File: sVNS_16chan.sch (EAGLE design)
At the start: 56 parts, among them IC2 OPA990IDCKR, IC3 EFM8SB10F2G-A-QFN20, J1 M50-3631042, J2 M50-3631042, J3 M50-3631042, U1 NT3H2211W0FHKH, U2 LT8410EDC-1#TRMPBF, U3 MUX36S16IRSNR, U4 MUX36S16IRSNR

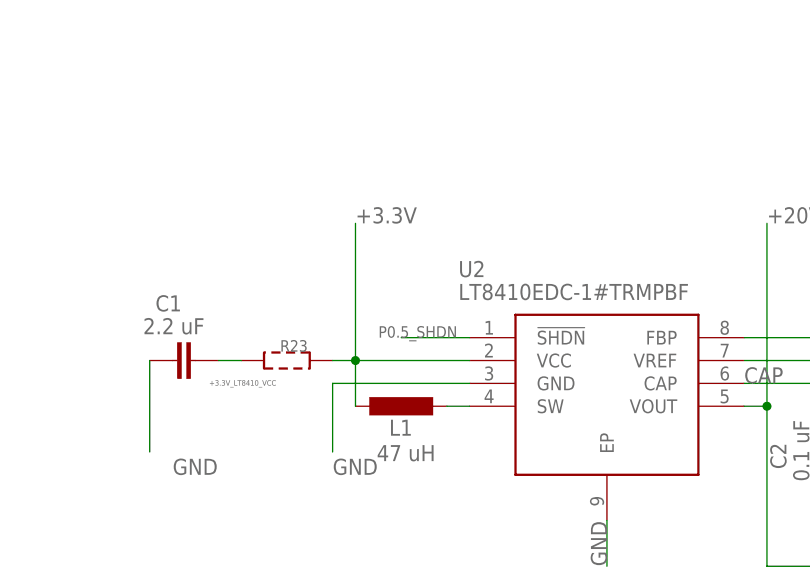
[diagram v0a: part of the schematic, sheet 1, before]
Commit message: Checkpoint 5. Closer to success?
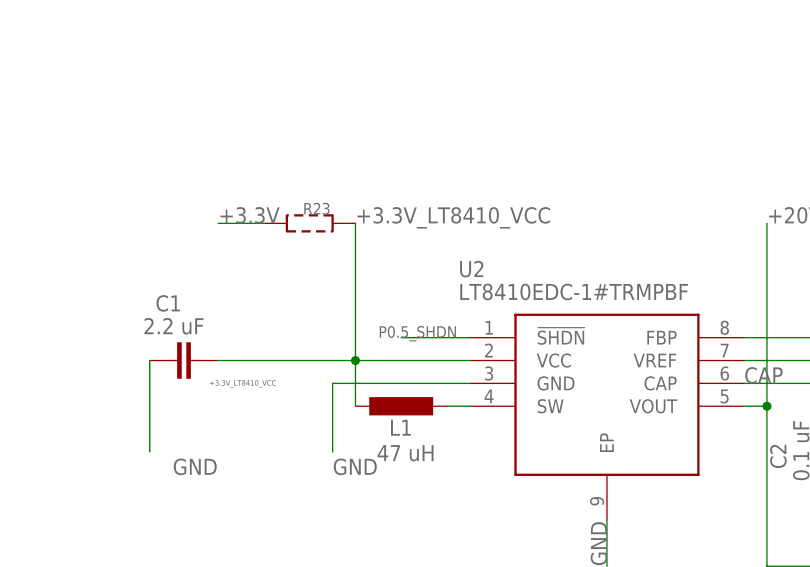
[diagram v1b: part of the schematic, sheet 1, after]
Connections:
- net +3.3V: now also R23.1; no longer L1.1, R23.2, U2.VCC
- net +3.3V_LT8410_VCC: now also L1.1, R23.2, U2.VCC; no longer R23.1
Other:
- moved on the sheet: R23
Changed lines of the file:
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@@
 <part name="R19" library="sVNS_16chan_lib" deviceset="SMD_PADS_0603" device="" package3d_urn="urn:adsk.eagle:package:23555/3"/>
 <part name="R20" library="sVNS_16chan_lib" deviceset="SMD_PADS_0603" device="" package3d_urn="urn:adsk.eagle:package:23555/3"/>
-<part name="R23" library="sVNS_16chan_lib" deviceset="SMD_PADS_0603" device="" package3d_urn="urn:adsk.eagle:package:23555/3"/>
 <part name="R24" library="sVNS_16chan_lib" deviceset="SMD_PADS_0603" device="" package3d_urn="urn:adsk.eagle:package:23555/3"/>
 <part name="R25" library="sVNS_16chan_lib" deviceset="SMD_PADS_0603" device="" package3d_urn="urn:adsk.eagle:package:23555/3"/>
@@
 <part name="R29" library="rcl" library_urn="urn:adsk.eagle:library:334" deviceset="R-EU_" device="R0402" package3d_urn="urn:adsk.eagle:package:23547/3" value="1.3M"/>
 <part name="R30" library="sVNS_16chan_lib" deviceset="SMD_PADS_0603" device="" package3d_urn="urn:adsk.eagle:package:23555/3"/>
+<part name="R23" library="sVNS_16chan_lib" deviceset="SMD_PADS_0603" device="" package3d_urn="urn:adsk.eagle:package:23555/3"/>
 </parts>
 <sheets>
@@
 <attribute name="VALUE" x="131.064" y="76.581" size="1.778" layer="96"/>
 </instance>
-<instance part="R23" gate="G$1" x="50.8" y="73.66" smashed="yes">
-<attribute name="NAME" x="50.038" y="74.6506" size="1.27" layer="95"/>
-<attribute name="VALUE" x="46.99" y="70.358" size="1.778" layer="96"/>
-</instance>
 <instance part="R24" gate="G$1" x="30.48" y="22.86" smashed="yes" rot="R90">
 <attribute name="NAME" x="29.4894" y="22.098" size="1.27" layer="95" rot="R90"/>
@@
 <attribute name="NAME" x="130.302" y="143.7894" size="1.27" layer="95" rot="R180"/>
 <attribute name="VALUE" x="133.35" y="148.082" size="1.778" layer="96" rot="R180"/>
+</instance>
+<instance part="R23" gate="G$1" x="53.34" y="88.9" smashed="yes">
+<attribute name="NAME" x="52.578" y="89.8906" size="1.27" layer="95"/>
+<attribute name="VALUE" x="49.53" y="85.598" size="1.778" layer="96"/>
 </instance>
 </instances>
@@
 </segment>
 <segment>
-<junction x="58.42" y="73.66"/>
-<wire x1="58.42" y1="73.66" x2="58.42" y2="88.9" width="0.1524" layer="91"/>
-<pinref part="L1" gate="G$1" pin="1"/>
-<wire x1="58.42" y1="68.58" x2="58.42" y2="73.66" width="0.1524" layer="91"/>
-<label x="58.42" y="88.9" size="1.778" layer="95"/>
-<pinref part="U2" gate="G$1" pin="VCC"/>
-<wire x1="58.42" y1="73.66" x2="71.12" y2="73.66" width="0.1524" layer="91"/>
-<wire x1="58.42" y1="73.66" x2="55.88" y2="73.66" width="0.1524" layer="91"/>
-<pinref part="R23" gate="G$1" pin="2"/>
-</segment>
-<segment>
 <pinref part="R26" gate="G$1" pin="2"/>
 <wire x1="10.16" y1="147.32" x2="10.16" y2="149.86" width="0.1524" layer="91"/>
 <label x="7.62" y="149.86" size="1.778" layer="95"/>
+</segment>
+<segment>
+<pinref part="R23" gate="G$1" pin="1"/>
+<wire x1="48.26" y1="88.9" x2="43.18" y2="88.9" width="0.1524" layer="91"/>
+<label x="43.18" y="88.9" size="1.778" layer="95"/>
 </segment>
 </net>
@@
 </segment>
 </net>
-<net name="+3.3V_LT8410_VCC" class="0">
-<segment>
-<pinref part="C1" gate="G$1" pin="2"/>
-<wire x1="43.18" y1="73.66" x2="45.72" y2="73.66" width="0.1524" layer="91"/>
-<pinref part="R23" gate="G$1" pin="1"/>
-<label x="42.164" y="70.866" size="0.6096" layer="95"/>
-</segment>
-</net>
 <net name="+3.3V_PIN" class="0">
 <segment>
@@
 </segment>
 </net>
+<net name="+3.3V_LT8410_VCC" class="0">
+<segment>
+<junction x="58.42" y="73.66"/>
+<wire x1="58.42" y1="73.66" x2="58.42" y2="88.9" width="0.1524" layer="91"/>
+<pinref part="L1" gate="G$1" pin="1"/>
+<wire x1="58.42" y1="68.58" x2="58.42" y2="73.66" width="0.1524" layer="91"/>
+<label x="58.42" y="88.9" size="1.778" layer="95"/>
+<pinref part="U2" gate="G$1" pin="VCC"/>
+<wire x1="58.42" y1="73.66" x2="71.12" y2="73.66" width="0.1524" layer="91"/>
+<pinref part="R23" gate="G$1" pin="2"/>
+<pinref part="C1" gate="G$1" pin="2"/>
+<label x="42.164" y="70.866" size="0.6096" layer="95"/>
+<wire x1="58.42" y1="73.66" x2="43.18" y2="73.66" width="0.1524" layer="91"/>
+</segment>
+</net>
